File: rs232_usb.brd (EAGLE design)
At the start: 40 x 40 mm, 17 parts, among them IC1 FT232RL, T1 BC847

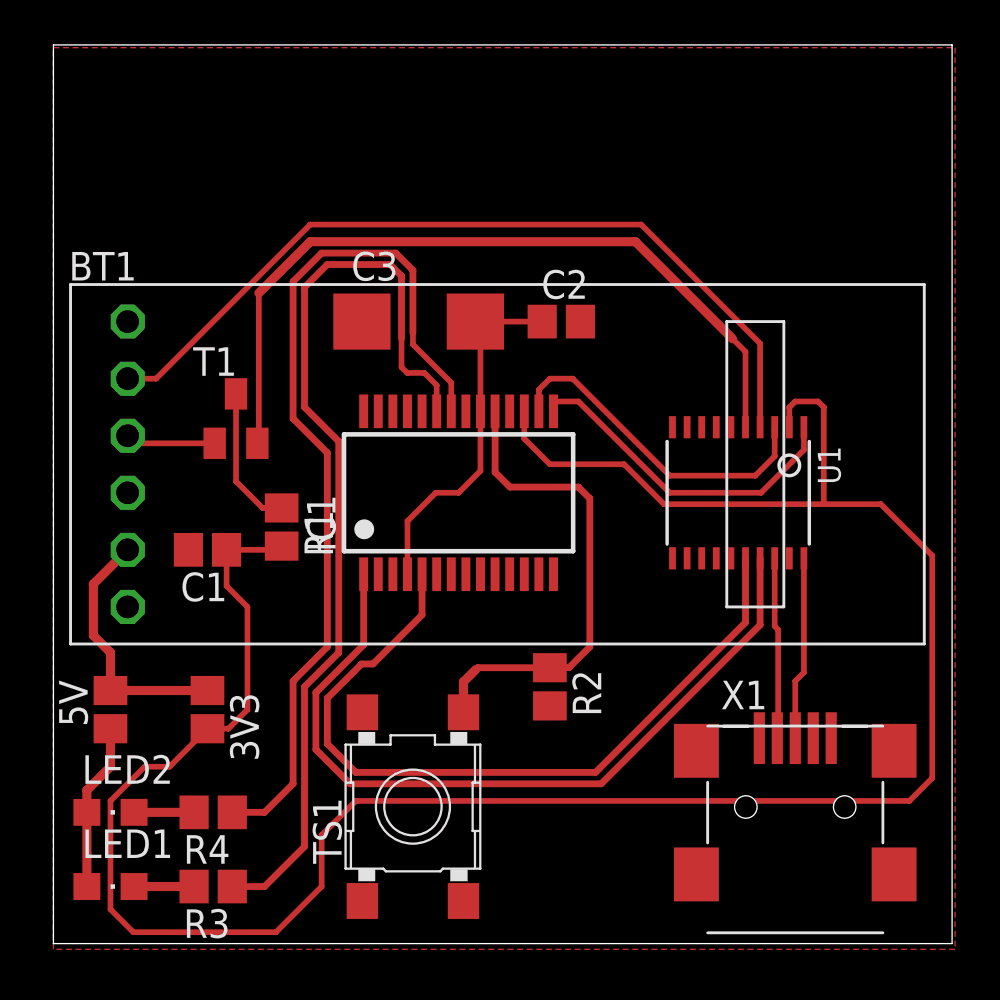
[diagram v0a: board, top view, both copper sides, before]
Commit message: 1. Fertiges Layout (Beidseitig)
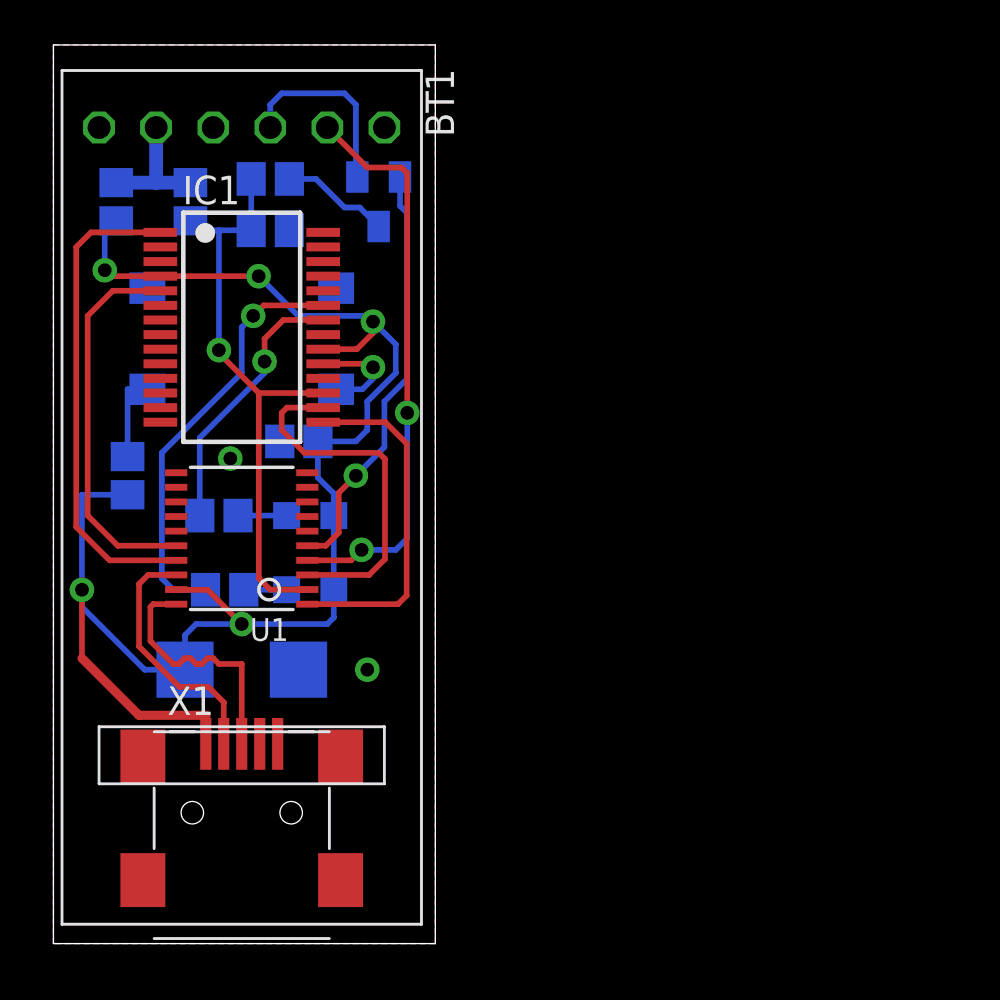
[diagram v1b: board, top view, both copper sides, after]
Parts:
- moved X1 24.6 mm to (8.38, 4.83)
- moved 3V3 22.6 mm to (6.10, 33.0), flipped to the bottom
- moved 5V 22.6 mm to (2.79, 33.0), flipped to the bottom
- moved U1 22.2 mm to (8.38, 18.0), turned to 90 degrees
- moved TS1 22.2 mm to (8.38, 26.9), flipped to the bottom, turned to 0 degrees
- moved R2 21.0 mm to (3.30, 20.8), flipped to the bottom
- moved C3 17.4 mm to (8.38, 12.2), flipped to the bottom
- moved LED2 15.9 mm to (11.4, 19.1), flipped to the bottom
- moved LED1 15.9 mm to (11.4, 15.7), flipped to the bottom
- moved BT1 15.8 mm to (8.38, 36.3), turned to 180 degrees
- moved R1 15.5 mm to (9.65, 34.0), flipped to the bottom, turned to 0 degrees
- moved C1 14.5 mm to (9.65, 31.8), flipped to the bottom
- moved R3 13.2 mm to (7.62, 15.7), flipped to the bottom
- moved R4 13.2 mm to (7.37, 19.1), flipped to the bottom
- moved C2 12.8 mm to (10.9, 22.4), flipped to the bottom
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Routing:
- net +3V3: track 102.6 -> 26.6 mm, vias 0 -> 1
- net +5V: track 23.8 -> 70.3 mm, vias 0 -> 5
- net LED2: track 40.0 -> 12.0 mm, vias 0 -> 1
- net LED1: track 42.2 -> 18.8 mm, vias 0 -> 1
- net RXD_5V: track 34.4 -> 17.1 mm
- net TXD_BT_3V3: track 34.7 -> 18.9 mm, vias 0 -> 1
- net TXD_5V: track 35.0 -> 21.5 mm
- net RESET: track 21.6 -> 8.50 mm, vias 0 -> 1
- net RXD_BT: track 36.9 -> 25.5 mm, vias 0 -> 2
- net N$1: track 11.5 -> 5.75 mm
- net TXD_BT: track 4.02 -> 8.49 mm
- net USB_5V_P: track 8.16 -> 11.2 mm
- net USB_5V_N: track 8.25 -> 11.2 mm
- net N$7: track 6.42 -> 4.85 mm
- net USB_3V3_N: track 15.1 -> 16.0 mm
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- added copper zone on layer 16, net GND
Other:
- board size 40 x 40 mm -> 17 x 40 mm
